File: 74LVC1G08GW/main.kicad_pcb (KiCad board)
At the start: 2 copper layers, 15.2 x 10.2 mm, 3 parts, among them P1 CONN_01X03, P2 CONN_01X03, U1 LM5050

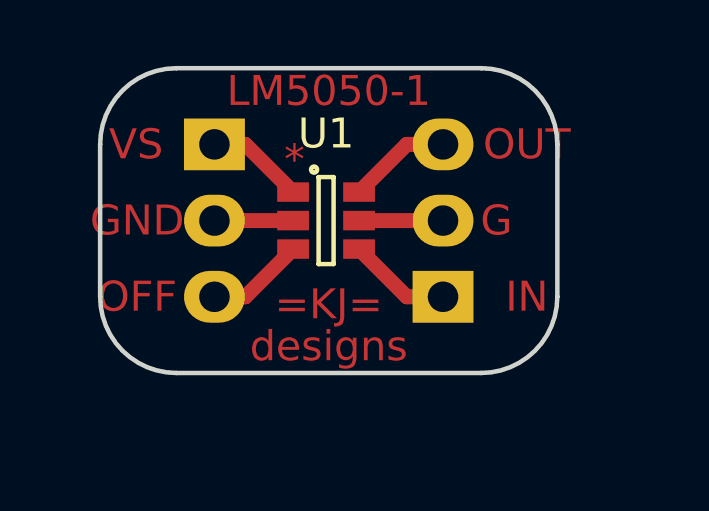
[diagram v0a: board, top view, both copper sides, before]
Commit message: test
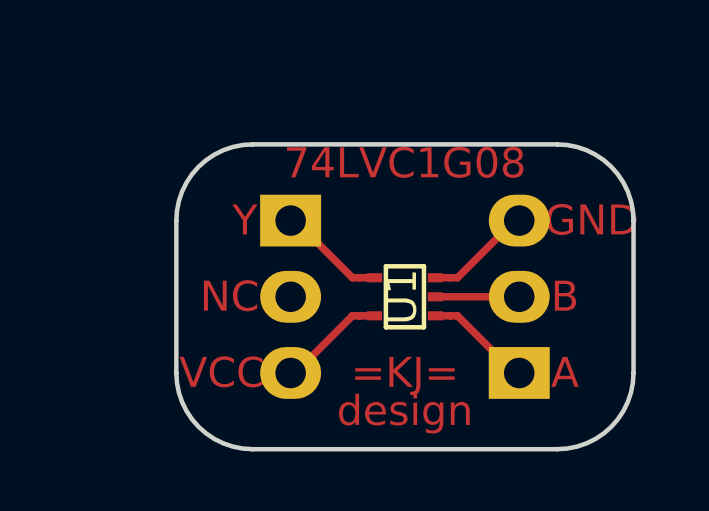
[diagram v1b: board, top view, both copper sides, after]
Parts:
- U1: value LM5050 -> 74LVC1G08; footprint TO_SOT_Packages_SMD:SOT-23-6 -> TO_SOT_Packages_SMD:SOT-353
- moved U1 3.66 mm to (151.1, 106.7), turned to 180 degrees
- moved P2 3.59 mm to (147.3, 104.1)
- moved P1 3.59 mm to (154.9, 109.2)
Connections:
- P2 pad 2: Net-(P2-Pad2) -> (no net)
- U1 pad 1: Net-(P2-Pad1) -> Net-(P1-Pad1)
- U1 pad 2: Net-(P2-Pad2) -> Net-(P1-Pad2)
- U1 pad 3: Net-(P2-Pad3) -> Net-(P1-Pad3)
- U1 pad 4: Net-(P1-Pad1) -> Net-(P2-Pad1)
- U1 pad 5: Net-(P1-Pad2) -> Net-(P2-Pad3)
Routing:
- net Net-(P2-Pad2): track 2.62 -> 0.00 mm
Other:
- board text added: "74LVC1G08"
- board text added: "A"
- board text added: "B"
- board text added: "NC"
- board text added: "VCC"
- board text added: "Y"
- board text added: "design"
- board text removed: "*"
- board text removed: "G"
- board text removed: "IN"
- board text removed: "LM5050-1"
- board text removed: "OFF"
- board text removed: "OUT"
- board text removed: "VS"
- board text removed: "designs"
